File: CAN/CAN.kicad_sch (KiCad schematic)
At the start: 24 parts, among them CN1 1.0T-4PLTPZ, J1 Conn_01x04, J2 Screw_Terminal_01x02, P1 USB_C_Plug_USB2.0, Q1 BSS214NW, Q2 BSS214NW, U1 AP2112K-3.3, U2 SN65HVD230, U5 ESP32-C3-MINI-1

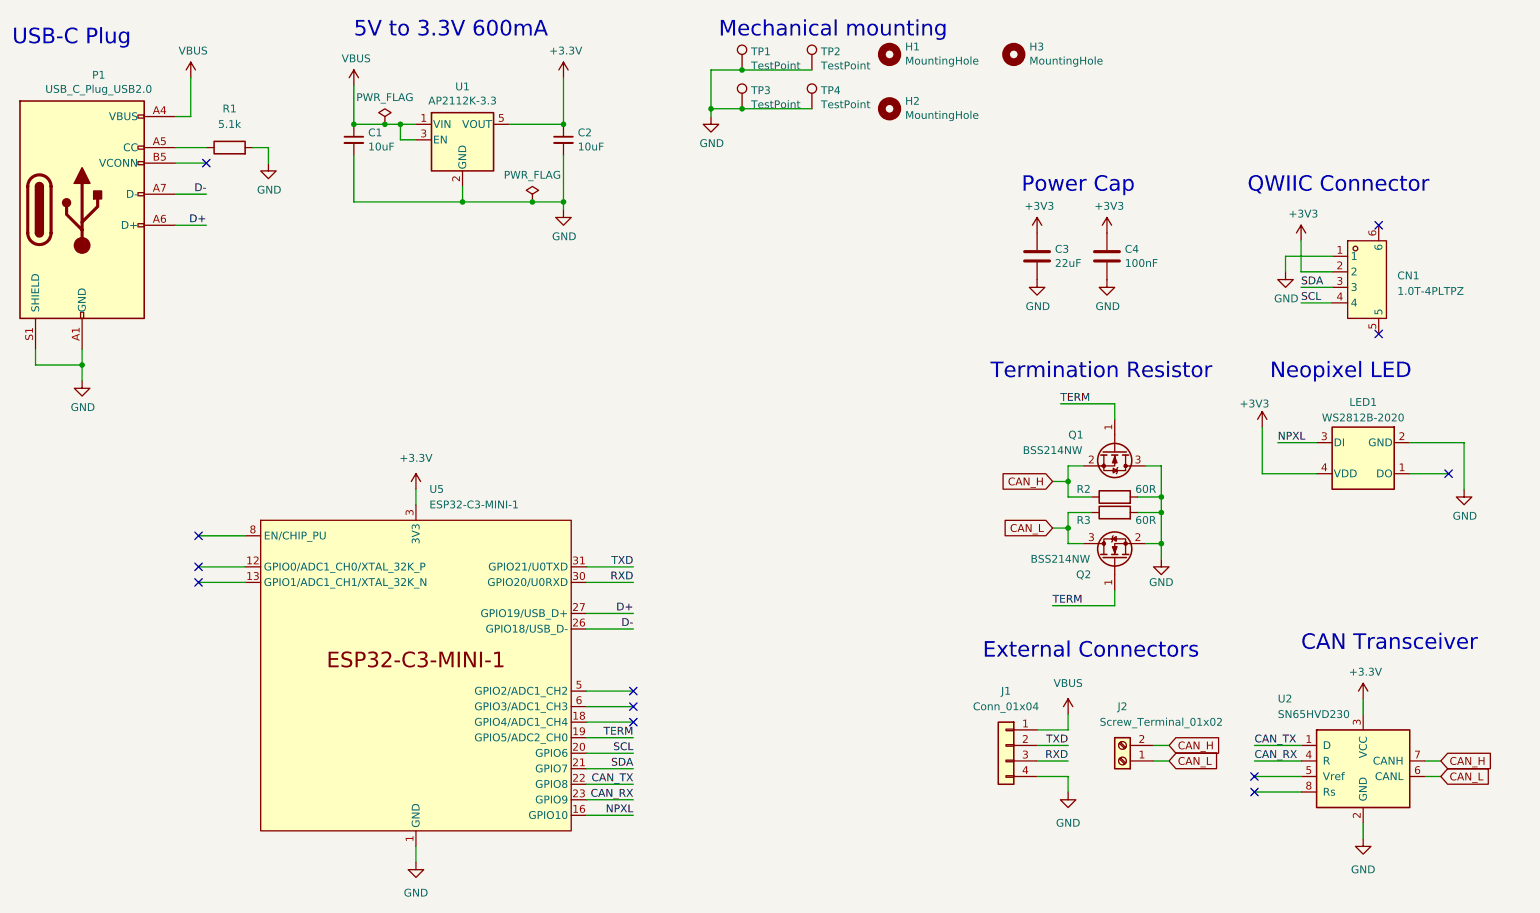
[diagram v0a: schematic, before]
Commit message: Cleaned Schematic
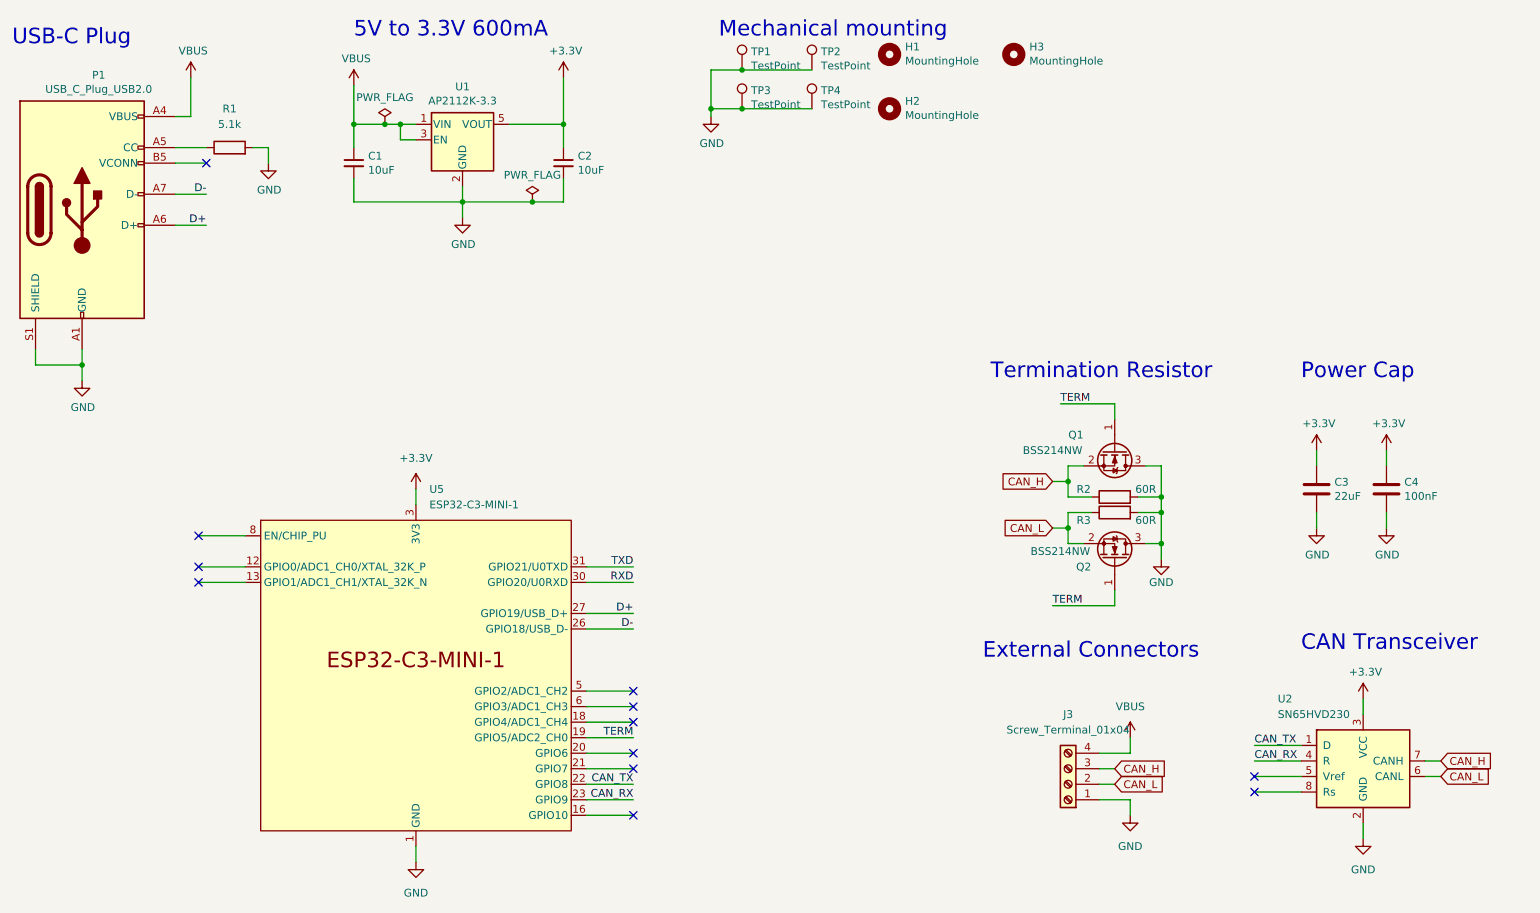
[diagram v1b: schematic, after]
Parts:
- removed CN1: 1.0T-4PLTPZ, _mykicadlib:FPC-SMD_4P-P1.00_1.0T-4PLTPZ, symbol _mykicadlib:QWIIC_1.0T-4PLTPZ
- removed J1: Conn_01x04, Connector_PinSocket_2.54mm:PinSocket_1x04_P2.54mm_Horizontal, symbol Connector_Generic:Conn_01x04
- removed J2: Screw_Terminal_01x02, Connector_PinHeader_2.54mm:PinHeader_1x02_P2.54mm_Horizontal, symbol Connector:Screw_Terminal_01x02
- removed LED1: WS2812B-2020, _mykicadlib:LED-SMD_4P-L2.0-W2.0-TL_WS2812B-2020, symbol _mykicadlib:WS2812B-2020
- added J3: Screw_Terminal_01x04, Connector_PinHeader_2.54mm:PinHeader_1x04_P2.54mm_Horizontal, symbol Connector:Screw_Terminal_01x04
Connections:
- net CAN_H: now also J3.3 (Pin_3)
- net CAN_L: now also Q2.2 (S), J3.2 (Pin_2); no longer Q2.3 (D)
- net GND: now also Q2.3 (D), J3.1 (Pin_1); no longer Q2.2 (S)
- net VBUS: now also J3.4 (Pin_4)
- net NPXL: no longer names the net of U5.16 (GPIO10)
- net SCL: no longer names the net of U5.20 (GPIO6)
- net SDA: no longer names the net of U5.21 (GPIO7)
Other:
- note removed: "Neopixel LED"
- note removed: "QWIIC Connector"
- moved on the sheet: C1, C2, C3, C4, Q2
